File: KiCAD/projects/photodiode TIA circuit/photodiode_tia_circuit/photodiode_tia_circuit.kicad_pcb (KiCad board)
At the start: 2 copper layers, 60 x 40 mm, 7 parts, among them P1 TO46_3PIN, U1 MCP6292

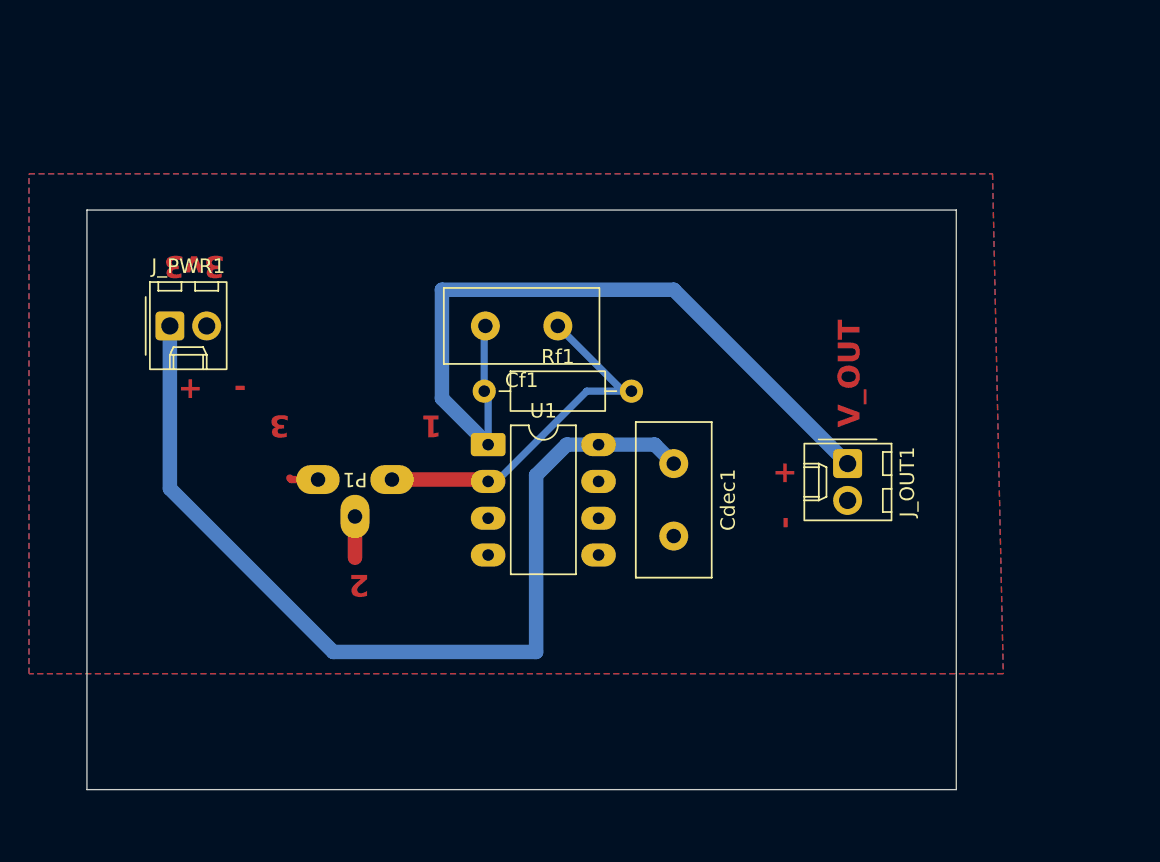
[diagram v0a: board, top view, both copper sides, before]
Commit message: manufacture documents and 3d model step file
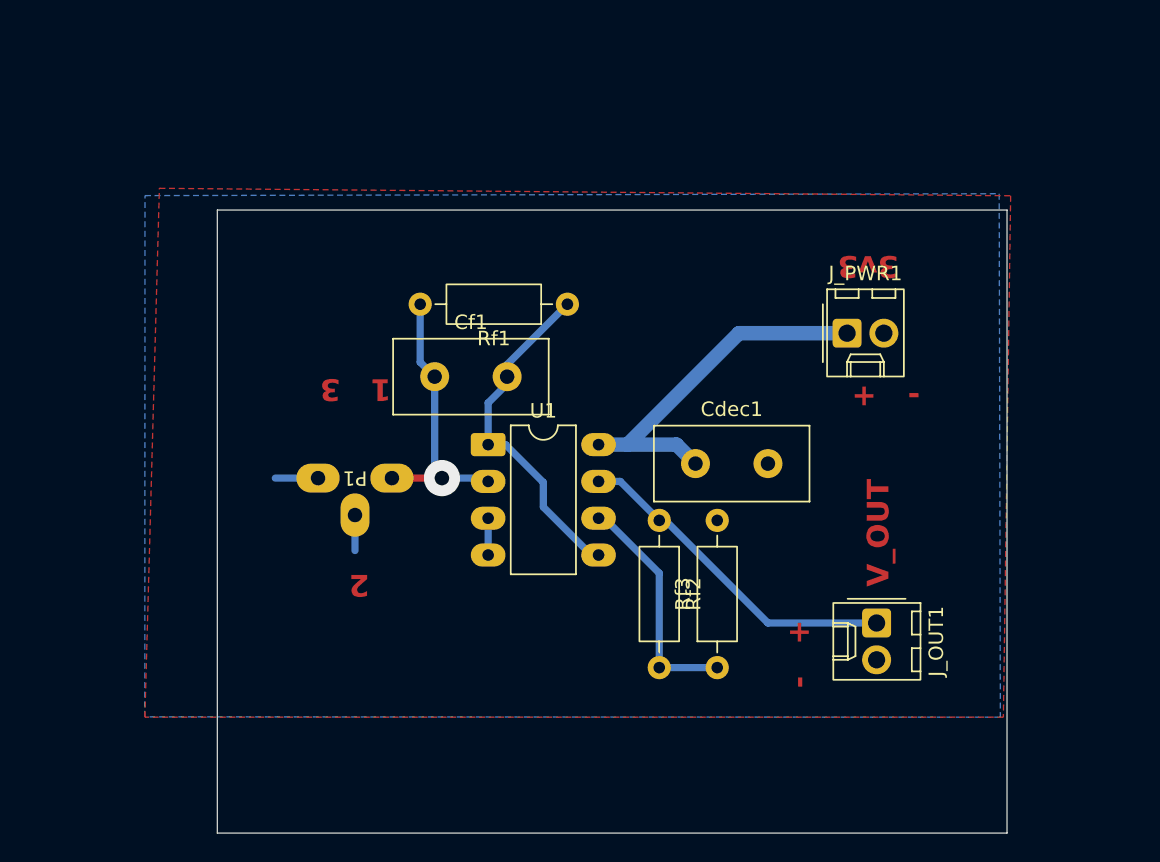
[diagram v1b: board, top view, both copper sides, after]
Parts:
- added Rf2: 100k, Resistor_THT:R_Axial_DIN0207_L6.3mm_D2.5mm_P10.16mm_Horizontal, F.Cu at (138.0, 84.9)
- added Rf3: 1.8k, Resistor_THT:R_Axial_DIN0207_L6.3mm_D2.5mm_P10.16mm_Horizontal, F.Cu at (142.0, 95.1)
- Cdec1: value 100nF -> 0.1uF
- Cf1: value DNP -> 2pF
- Rf1: value 10M R -> 470k
- moved J_PWR1 46.7 mm to (151.0, 72.0)
- moved J_OUT1 11.2 mm to (153.0, 92.0)
- moved Cf1 9.19 mm to (122.5, 75.0), turned to 0 degrees
- moved Rf1 8.30 mm to (131.7, 70.0), turned to 180 degrees
- moved Cdec1 1.50 mm to (140.5, 81.0), turned to 0 degrees
- moved P1 0.10 mm to (117.0, 82.0)
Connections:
- Cf1 pad 2: Net-(J_OUT1-Pin_1) -> Net-(U1B-+)
- Rf1 pad 1: Net-(J_OUT1-Pin_1) -> Net-(U1B-+)
- U1 pad 1: Net-(J_OUT1-Pin_1) -> Net-(U1B-+)
- U1 pad 5: GND -> Net-(U1B-+)
- U1 pad 6: GND -> Net-(U1B--)
- U1 pad 7: GND -> Net-(J_OUT1-Pin_1)
- U1 pad 8: (no net) -> +3.3V
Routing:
- net +3.3V: track 64.3 -> 27.8 mm
- net Net-(J_OUT1-Pin_1): track 53.3 -> 23.2 mm
- net Net-(U1B-+): track 0.00 -> 23.7 mm
- net Net-(U1B--): track 0.00 -> 16.3 mm
- net Net-(P1-Cathode): track 26.1 -> 19.4 mm, vias 0 -> 1
- net GND: track 5.16 -> 7.94 mm
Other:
- board size 60 x 40 mm -> 54.5 x 43 mm

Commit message: new
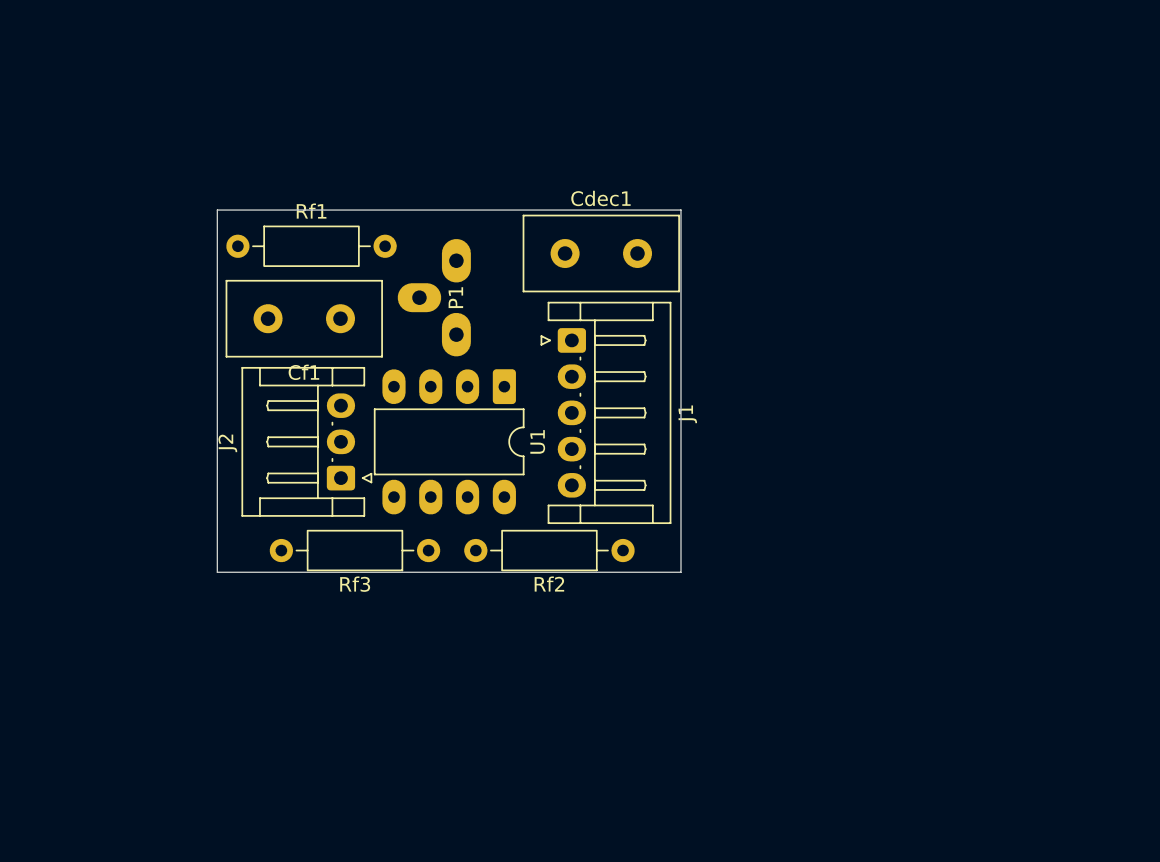
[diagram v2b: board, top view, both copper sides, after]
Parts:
- removed J_OUT1, J_PWR1: Conn_01x02_Socket, Connector_Molex:Molex_KK-254_AE-6410-02A_1x02_P2.54mm_Vertical
- added J1: Conn_01x05_Socket, Connector_JST:JST_EH_S5B-EH_1x05_P2.50mm_Horizontal, F.Cu at (132.0, 72.5)
- added J2: Conn_01x03_Socket, Connector_JST:JST_EH_S3B-EH_1x03_P2.50mm_Horizontal, F.Cu at (116.0, 82.0)
- moved Rf1 23.1 mm to (108.9, 66.0), turned to 0 degrees
- moved Rf3 21.5 mm to (122.1, 87.0), turned to 180 degrees
- moved Cdec1 17.1 mm to (131.5, 66.5)
- moved P1 14.3 mm to (124.0, 69.5), turned to 90 degrees
- moved Cf1 7.63 mm to (116.0, 71.0), turned to 180 degrees
- moved U1 4.15 mm to (127.3, 75.7), turned to -90 degrees
- moved Rf2 3.25 mm to (135.5, 87.0), turned to 180 degrees
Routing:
- net +3.3V: track 27.8 -> 0.00 mm
- net Net-(U1B-+): track 23.7 -> 0.00 mm
- net Net-(J1-Pin_3): track 23.2 -> 0.00 mm
- net Net-(P1-Cathode): track 19.4 -> 0.00 mm, vias 1 -> 0
- net Net-(U1B--): track 16.3 -> 0.00 mm
- net GND: track 7.94 -> 0.00 mm
- removed copper zone on B.Cu, net GND
- removed copper zone on F.Cu, net GND
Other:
- board size 54.5 x 43 mm -> 32 x 25 mm
- board text removed: "- +"
- board text removed: "1"
- board text removed: "2"
- board text removed: "3"
- board text removed: "3v3"
- board text removed: "V_OUT"

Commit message: latest version
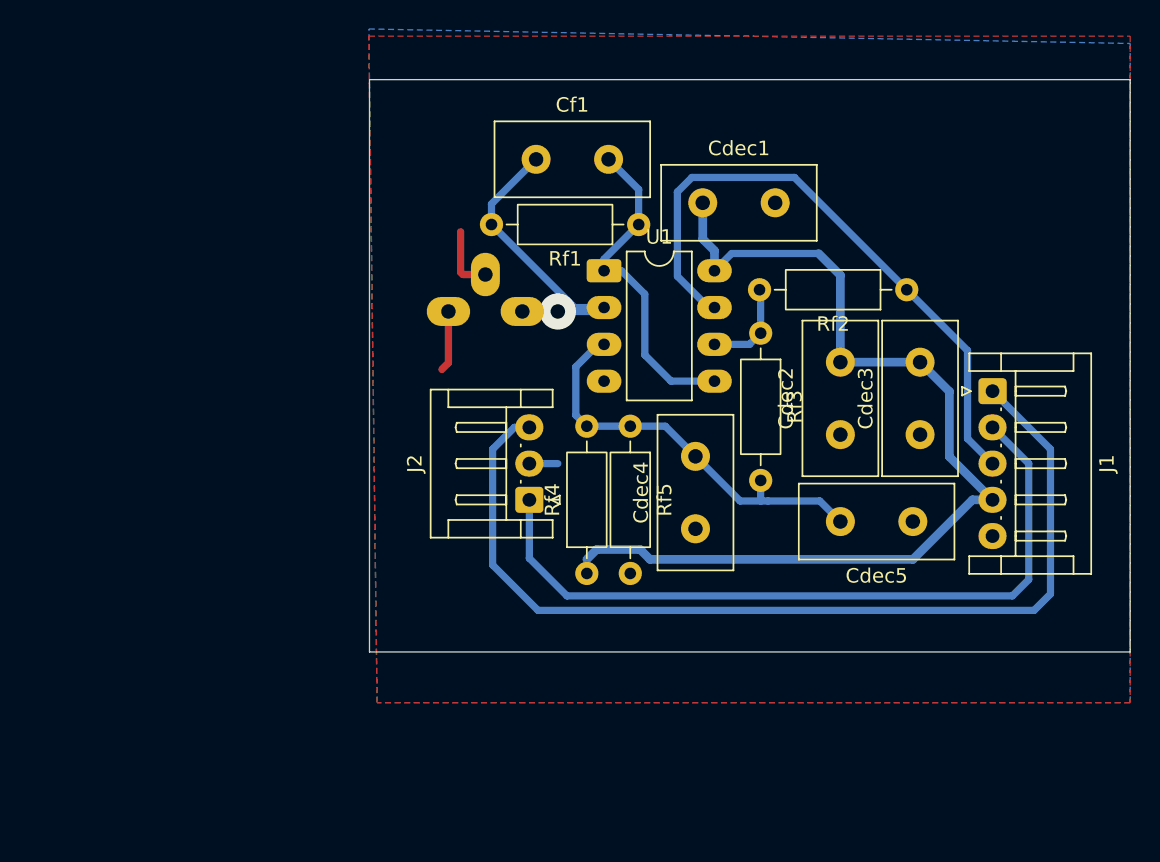
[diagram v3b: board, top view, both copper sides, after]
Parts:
- added Cdec2: 10uF, Capacitor_THT:C_Disc_D10.5mm_W5.0mm_P5.00mm, F.Cu at (150.5, 79.0)
- added Cdec3: 100nF, Capacitor_THT:C_Disc_D10.5mm_W5.0mm_P5.00mm, F.Cu at (156.0, 79.0)
- added Cdec4: 100nF, Capacitor_THT:C_Disc_D10.5mm_W5.0mm_P5.00mm, F.Cu at (140.5, 85.5)
- added Cdec5: 10uF, Capacitor_THT:C_Disc_D10.5mm_W5.0mm_P5.00mm, F.Cu at (155.5, 85.0)
- added Rf4: 5.6k, Resistor_THT:R_Axial_DIN0207_L6.3mm_D2.5mm_P10.16mm_Horizontal, F.Cu at (133.0, 88.6)
- added Rf5: 1k, Resistor_THT:R_Axial_DIN0207_L6.3mm_D2.5mm_P10.16mm_Horizontal, F.Cu at (136.0, 78.4)
- Cdec1: value 0.1uF -> 100nF
- P1: moved to B.Cu
- moved J1 29.2 mm to (161.0, 76.0)
- moved Rf1 27.7 mm to (136.6, 64.5), turned to 180 degrees
- moved Rf3 27.4 mm to (145.0, 72.0), turned to -90 degrees
- moved Rf2 26.6 mm to (155.1, 69.0)
- moved Cf1 17.4 mm to (129.5, 60.0), turned to 0 degrees
- moved J2 13.1 mm to (129.0, 83.5)
- moved U1 10.6 mm to (134.2, 67.7), turned to 0 degrees
- moved Cdec1 10.1 mm to (141.0, 63.0)
- moved P1 2.21 mm to (126.0, 70.5), turned to 180 degrees
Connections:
- Rf3 pad 2: GND -> Net-(U1A-+)
- U1 pad 3: GND -> Net-(U1A-+)
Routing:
- net +3.3V: track 0.00 -> 68.2 mm
- net Net-(J1-Pin_1): track 0.00 -> 67.1 mm
- net Net-(J1-Pin_2): track 0.00 -> 51.6 mm
- net Net-(J1-Pin_3): track 0.00 -> 43.2 mm
- net Net-(U1A-+): track 0.00 -> 28.7 mm
- net Net-(U1B-+): track 0.00 -> 22.8 mm
- net Net-(P1-Cathode): track 0.00 -> 21.7 mm, vias 0 -> 1
- net GND: track 0.00 -> 10.7 mm
- net Net-(U1B--): track 0.00 -> 6.54 mm
- added copper zone on B.Cu, net GND
- added copper zone on F.Cu, net GND
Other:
- board size 32 x 25 mm -> 52.5 x 39.5 mm
